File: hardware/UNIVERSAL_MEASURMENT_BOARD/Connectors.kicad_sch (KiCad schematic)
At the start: 17 parts, among them J1 2604-1104, J10 2604-1104, J11 2604-1104, J12 2604-1104, J13 2604-1104, J14 2604-1104, J15 2604-1104, J16 2604-1104, J17 2604-1104, J2 2604-1104, J3 2604-1104, J4 2604-1104, J5 2604-1104, J6 2604-1104, J7 2604-1104, J8 2604-1104, J9 2604-1104

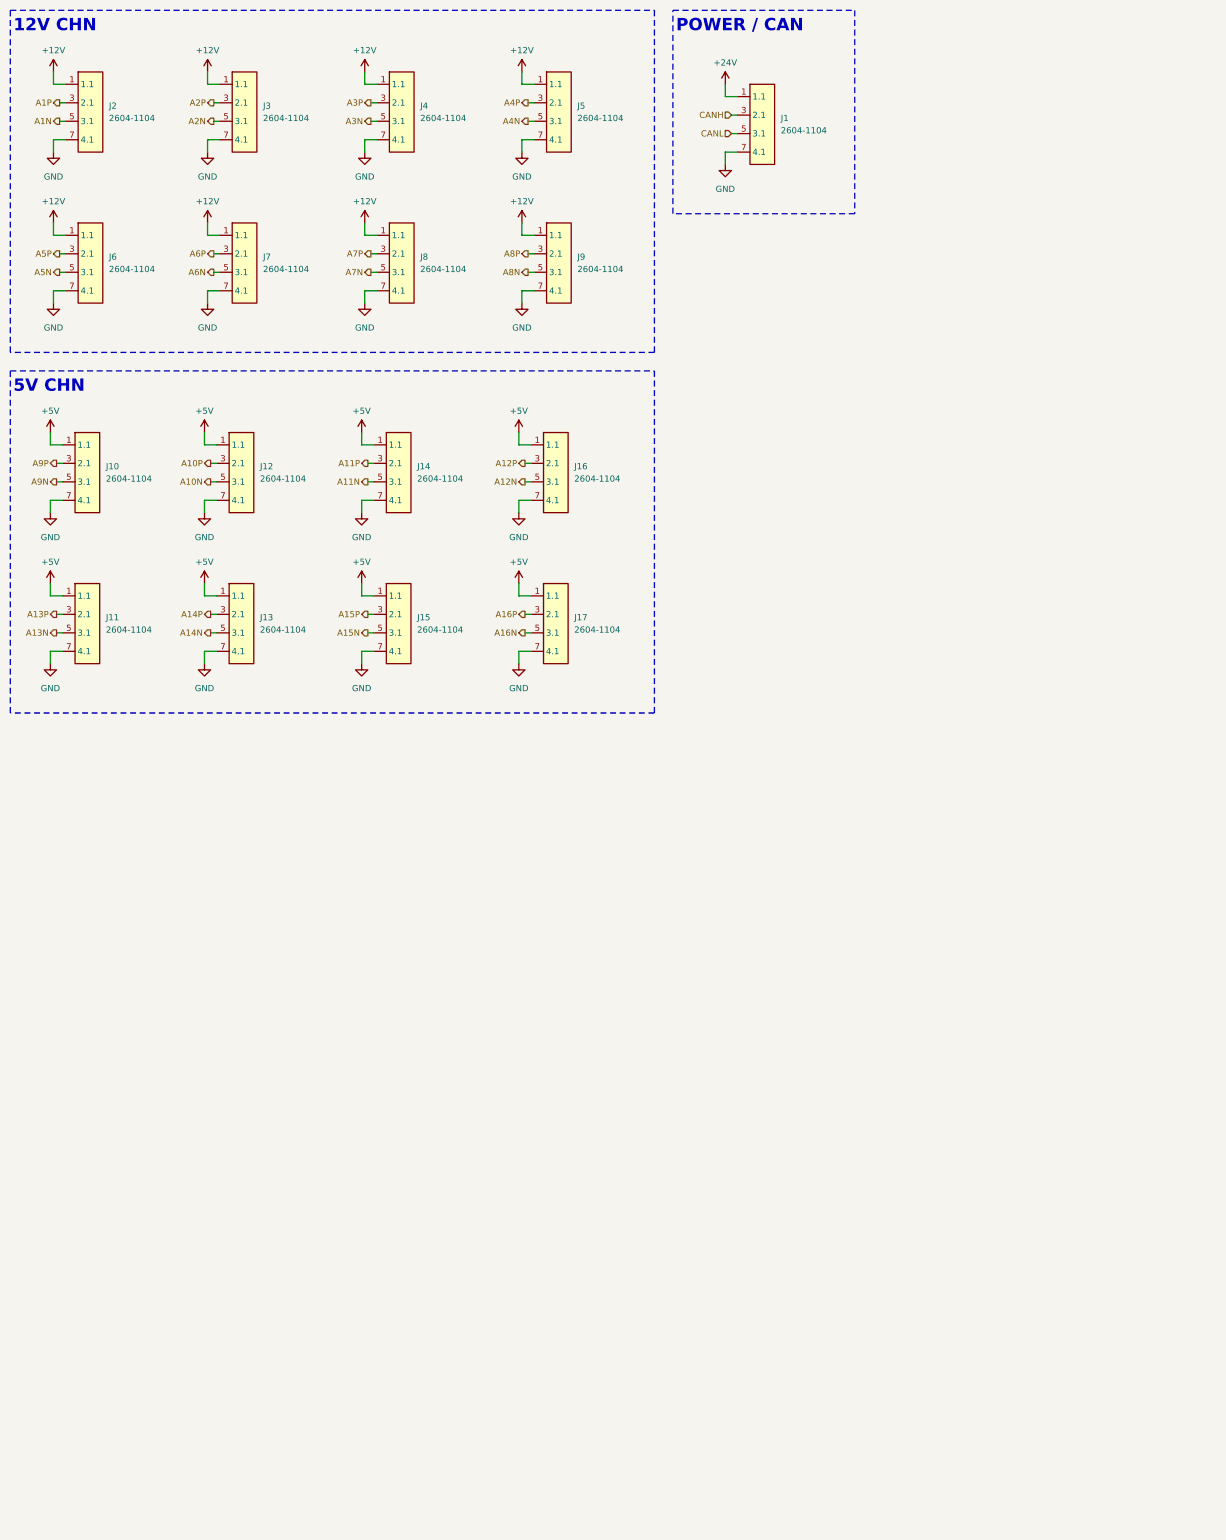
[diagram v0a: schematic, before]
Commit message: continued
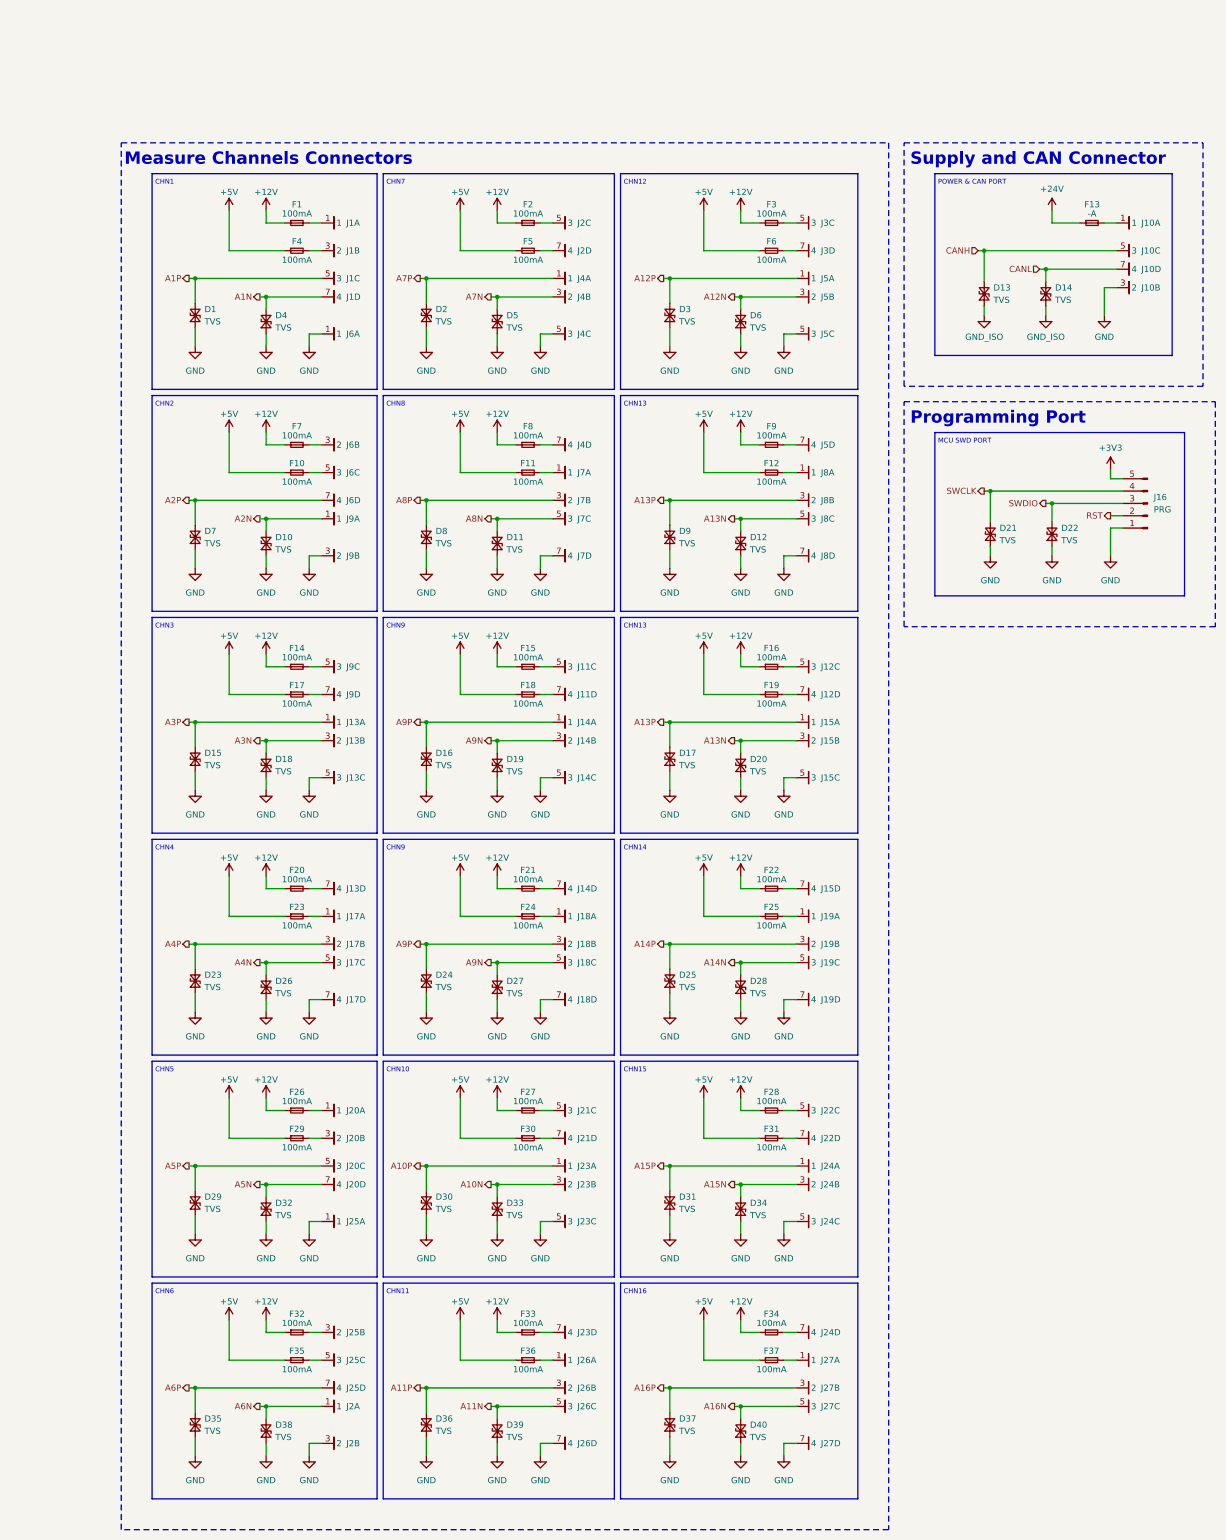
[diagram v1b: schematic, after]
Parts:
- removed J11, J12, J16, J3: 2604-1104, 26041104, symbol 2604-1104:2604-1104
- added D1, D10, D11, D12, D13, D14, D15, D16, D17, D18, D19, D2, D20, D21, D22, D23, D24, D25, D26, D27, D28, D29, D3, D30, D31, D32, D33, D34, D35, D36, D37, D38, D39, D4, D40, D5, D6, D7, D8, D9: TVS, symbol Device:D_TVS_Small
- added F1, F10, F11, F12, F14, F15, F16, F17, F18, F19, F2, F20, F21, F22, F23, F24, F25, F26, F27, F28, F29, F3, F30, F31, F32, F33, F34, F35, F36, F37, F4, F5, F6, F7, F8, F9: 100mA, symbol Device:Fuse_Small
- added F13: -A, symbol Device:Fuse_Small
- added unit 3 of J1
- added unit 4 of J1
- added unit 2 of J1
- added unit 2 of J10
- added unit 3 of J10
- added unit 4 of J10
- added J11, J12, J18, J19, J20, J21, J22, J23, J24, J25, J26, J27, J3: 2604-1104, 26041104, symbol 2604-1104:2604-1104
- added unit 4 of J13
- added unit 2 of J13
- added unit 3 of J13
- added unit 3 of J14
- added unit 2 of J14
- added unit 4 of J14
- added unit 4 of J15
- added unit 3 of J15
- added unit 2 of J15
- added J16: PRG, Connector_PinHeader_1.00mm:PinHeader_1x05_P1.00mm_Vertical, symbol Connector:Conn_01x05_Pin
- added unit 3 of J17
- added unit 4 of J17
- added unit 2 of J17
- added unit 4 of J2
- added unit 2 of J2
- added unit 3 of J2
- added unit 4 of J4
- added unit 2 of J4
- added unit 3 of J4
- added unit 4 of J5
- added unit 2 of J5
- added unit 3 of J5
- added unit 3 of J6
- added unit 4 of J6
- added unit 2 of J6
- added unit 4 of J7
- added unit 2 of J7
- added unit 3 of J7
- added unit 4 of J8
- added unit 3 of J8
- added unit 2 of J8
- added unit 4 of J9
- added unit 3 of J9
- added unit 2 of J9
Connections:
- net +12V: now also F1.1, F14.1, F15.1, F16.1, F2.1, F20.1, F21.1, F22.1, F26.1, F27.1, F28.1, F3.1, F32.1, F33.1, F34.1, F7.1, F8.1, F9.1; no longer J2.1 (1.1), J2.2 (1.2), J4.1 (1.1), J4.2 (1.2), J5.1 (1.1), J5.2 (1.2), J6.1 (1.1), J6.2 (1.2), J7.1 (1.1), J7.2 (1.2), J8.1 (1.1), J8.2 (1.2), J9.1 (1.1), J9.2 (1.2)
- net +24V: now also F13.1; no longer J1.1 (1.1), J1.2 (1.2)
- net +5V: now also F10.1, F11.1, F12.1, F17.1, F18.1, F19.1, F23.1, F24.1, F25.1, F29.1, F30.1, F31.1, F35.1, F36.1, F37.1, F4.1, F5.1, F6.1; no longer J10.1 (1.1), J10.2 (1.2), J13.1 (1.1), J13.2 (1.2), J14.1 (1.1), J14.2 (1.2), J15.1 (1.1), J15.2 (1.2), J17.1 (1.1), J17.2 (1.2)
- net A10N: now also D33.2 (A2), J23.3 (2), J23.4 (2.2)
- net A10P: now also D30.2 (A2), J23.1, J23.2 (1.2)
- net A11N: now also D39.2 (A2), J26.5 (3), J26.6 (3.2); no longer J14.5 (3.1), J14.6 (3.2)
- net A11P: now also D36.2 (A2), J26.3 (2), J26.4 (2.2); no longer J14.3 (2.1), J14.4 (2.2)
- net A12N: now also D6.2 (A2), J5.3 (2), J5.4 (2.2)
- net A12P: now also J5.1, J5.2 (1.2), D3.2 (A2)
- net A13N: now also D12.2 (A2), D20.2 (A2), J15.3 (2), J15.4 (2.2), J8.5 (3), J8.6 (3.2)
- net A13P: now also J15.1, J15.2 (1.2), D17.2 (A2), D9.2 (A2), J8.3 (2), J8.4 (2.2)
- net A14N: now also D28.2 (A2), J19.5 (3), J19.6 (3.2); no longer J13.5 (3.1), J13.6 (3.2)
- net A14P: now also D25.2 (A2), J19.3 (2), J19.4 (2.2); no longer J13.3 (2.1), J13.4 (2.2)
- net A15N: now also D34.2 (A2), J24.3 (2), J24.4 (2.2); no longer J15.5 (3.1), J15.6 (3.2)
- net A15P: now also D31.2 (A2), J24.1, J24.2 (1.2); no longer J15.3 (2.1), J15.4 (2.2)
- net A16N: now also D40.2 (A2), J27.5 (3), J27.6 (3.2); no longer J17.5 (3.1), J17.6 (3.2)
- net A16P: now also D37.2 (A2), J27.3 (2), J27.4 (2.2); no longer J17.3 (2.1), J17.4 (2.2)
- net A1N: now also D4.2 (A2), J1.7 (4), J1.8 (4.2); no longer J2.5 (3.1), J2.6 (3.2)
- net A1P: now also D1.2 (A2), J1.5 (3), J1.6 (3.2); no longer J2.3 (2.1), J2.4 (2.2)
- net A2N: now also J9.1, J9.2 (1.2), D10.2 (A2)
- net A2P: now also D7.2 (A2), J6.7 (4), J6.8 (4.2)
- net A3N: now also D18.2 (A2), J13.3 (2), J13.4 (2.2); no longer J4.5 (3.1), J4.6 (3.2)
- net A3P: now also J13.1, J13.2 (1.2), D15.2 (A2); no longer J4.3 (2.1), J4.4 (2.2)
- net A4N: now also D26.2 (A2), J17.5 (3), J17.6 (3.2); no longer J5.5 (3.1), J5.6 (3.2)
- net A4P: now also D23.2 (A2), J17.3 (2), J17.4 (2.2); no longer J5.3 (2.1), J5.4 (2.2)
- net A5N: now also D32.2 (A2), J20.7 (4), J20.8 (4.2); no longer J6.5 (3.1), J6.6 (3.2)
- net A5P: now also D29.2 (A2), J20.5 (3), J20.6 (3.2); no longer J6.3 (2.1), J6.4 (2.2)
- net A6N: now also J2.1, J2.2 (1.2), D38.2 (A2); no longer J7.5 (3.1), J7.6 (3.2)
- net A6P: now also D35.2 (A2), J25.7 (4), J25.8 (4.2); no longer J7.3 (2.1), J7.4 (2.2)
- net A7N: now also D5.2 (A2), J4.3 (2), J4.4 (2.2); no longer J8.5 (3.1), J8.6 (3.2)
- net A7P: now also J4.1, J4.2 (1.2), D2.2 (A2); no longer J8.3 (2.1), J8.4 (2.2)
- net A8N: now also D11.2 (A2), J7.5 (3), J7.6 (3.2); no longer J9.5 (3.1), J9.6 (3.2)
- net A8P: now also D8.2 (A2), J7.3 (2), J7.4 (2.2); no longer J9.3 (2.1), J9.4 (2.2)
- net A9N: now also D19.2 (A2), D27.2 (A2), J14.3 (2), J14.4 (2.2), J18.5 (3), J18.6 (3.2); no longer J10.5 (3.1), J10.6 (3.2)
- net A9P: now also J14.1, J14.2 (1.2), D16.2 (A2), D24.2 (A2), J18.3 (2), J18.4 (2.2); no longer J10.3 (2.1), J10.4 (2.2)
- net CANH: now also D13.2 (A2), J10.5 (3), J10.6 (3.2); no longer J1.3 (2.1), J1.4 (2.2)
- net CANL: now also D14.2 (A2), J10.7 (4), J10.8 (4.2); no longer J1.5 (3.1), J1.6 (3.2)
- net GND: now also J6.1, J6.2 (1.2), D1.1 (A1), D10.1 (A1), D11.1 (A1), D12.1 (A1), D15.1 (A1), D16.1 (A1), D17.1 (A1), D18.1 (A1), D19.1 (A1), D2.1 (A1), D20.1 (A1), D21.1 (A1), D22.1 (A1), D23.1 (A1), D24.1 (A1), D25.1 (A1), D26.1 (A1), D27.1 (A1), D28.1 (A1), D29.1 (A1), D3.1 (A1), D30.1 (A1), D31.1 (A1), D32.1 (A1), D33.1 (A1), D34.1 (A1), D35.1 (A1), D36.1 (A1), D37.1 (A1), D38.1 (A1), D39.1 (A1), D4.1 (A1), D40.1 (A1), D5.1 (A1), D6.1 (A1), D7.1 (A1), D8.1 (A1), D9.1 (A1), J10.3 (2), J10.4 (2.2), J13.5 (3), J13.6 (3.2), J14.5 (3), J14.6 (3.2), J15.5 (3), J15.6 (3.2), J16.1 (Pin_1), J17.7 (4), J17.8 (4.2), J18.7 (4), J18.8 (4.2), J19.7 (4), J19.8 (4.2), J2.3 (2), J2.4 (2.2), J23.5 (3), J23.6 (3.2), J24.5 (3), J24.6 (3.2), J25.1, J25.2 (1.2), J26.7 (4), J26.8 (4.2), J27.7 (4), J27.8 (4.2), J4.5 (3), J4.6 (3.2), J5.5 (3), J5.6 (3.2), J7.7 (4), J7.8 (4.2), J8.7 (4), J8.8 (4.2), J9.3 (2), J9.4 (2.2); no longer J1.7 (4.1), J1.8 (4.2), J10.7 (4.1), J10.8 (4.2), J13.7 (4.1), J13.8 (4.2), J14.7 (4.1), J14.8 (4.2), J15.7 (4.1), J15.8 (4.2), J17.7 (4.1), J17.8 (4.2), J2.7 (4.1), J2.8 (4.2), J4.7 (4.1), J4.8 (4.2), J5.7 (4.1), J5.8 (4.2), J6.7 (4.1), J6.8 (4.2), J7.7 (4.1), J7.8 (4.2), J8.7 (4.1), J8.8 (4.2), J9.7 (4.1), J9.8 (4.2)
- new net: F28.2, J22.5 (3), J22.6 (3.2)
- new net: F13.2, J10.1, J10.2 (1.2)
- new net: F19.2, J12.7 (4), J12.8 (4.2)
- new net: F9.2, J5.7 (4), J5.8 (4.2)
- new net: F11.2, J7.1, J7.2 (1.2)
- new net: F12.2, J8.1, J8.2 (1.2)
- new net: F30.2, J21.7 (4), J21.8 (4.2)
- new net: F24.2, J18.1, J18.2 (1.2)
- new net: F35.2, J25.5 (3), J25.6 (3.2)
- new net: F10.2, J6.5 (3), J6.6 (3.2)
- new net: F1.2, J1.1, J1.2 (1.2)
- new net: F8.2, J4.7 (4), J4.8 (4.2)
- new net: F22.2, J15.7 (4), J15.8 (4.2)
- new net: F20.2, J13.7 (4), J13.8 (4.2)
- new net: F5.2, J2.7 (4), J2.8 (4.2)
- new net: F32.2, J25.3 (2), J25.4 (2.2)
- new net: F3.2, J3.5 (3), J3.6 (3.2)
- new net: F31.2, J22.7 (4), J22.8 (4.2)
- new net: F25.2, J19.1, J19.2 (1.2)
- new net: F15.2, J11.5 (3), J11.6 (3.2)
- new net: F26.2, J20.1, J20.2 (1.2)
- new net: F33.2, J23.7 (4), J23.8 (4.2)
- new net: F36.2, J26.1, J26.2 (1.2)
- new net: F4.2, J1.3 (2), J1.4 (2.2)
- new net: F37.2, J27.1, J27.2 (1.2)
- new net: F27.2, J21.5 (3), J21.6 (3.2)
- new net: F23.2, J17.1, J17.2 (1.2)
- new net: F2.2, J2.5 (3), J2.6 (3.2)
- new net: F17.2, J9.7 (4), J9.8 (4.2)
- new net: F29.2, J20.3 (2), J20.4 (2.2)
- new net: F34.2, J24.7 (4), J24.8 (4.2)
- new net: F14.2, J9.5 (3), J9.6 (3.2)
- new net: F7.2, J6.3 (2), J6.4 (2.2)
- new net: F16.2, J12.5 (3), J12.6 (3.2)
- new net: F21.2, J14.7 (4), J14.8 (4.2)
- new net: F6.2, J3.7 (4), J3.8 (4.2)
- new net: F18.2, J11.7 (4), J11.8 (4.2)
- new net +3V3: J16.5 (Pin_5)
- new net GND_ISO: D13.1 (A1), D14.1 (A1)
- new net RST: J16.2 (Pin_2)
- new net SWCLK: D21.2 (A2), J16.4 (Pin_4)
- new net SWDIO: D22.2 (A2), J16.3 (Pin_3)
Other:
- note added: "CHN1"
- note added: "CHN10"
- note added: "CHN11"
- note added: "CHN12"
- note added: "CHN13"
- note added: "CHN14"
- note added: "CHN15"
- note added: "CHN16"
- note added: "CHN2"
- note added: "CHN3"
- note added: "CHN4"
- note added: "CHN5"
- note added: "CHN6"
- note added: "CHN7"
- note added: "CHN8"
- note added: "CHN9"
- note added: "MCU SWD PORT"
- note added: "Measure Channels Connectors"
- note added: "POWER & CAN PORT"
- note added: "Programming Port"
- note added: "Supply and CAN Connector"
- note removed: "12V CHN"
- note removed: "5V CHN"
- note removed: "POWER / CAN"
- company: (none) -> PUT Motorsport Formula Student team
- title: (none) -> Universal Measurment Board
